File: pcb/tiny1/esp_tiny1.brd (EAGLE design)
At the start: 45 x 95 mm, 35 parts, among them IC1 4000D, Q1 BUZ11BH

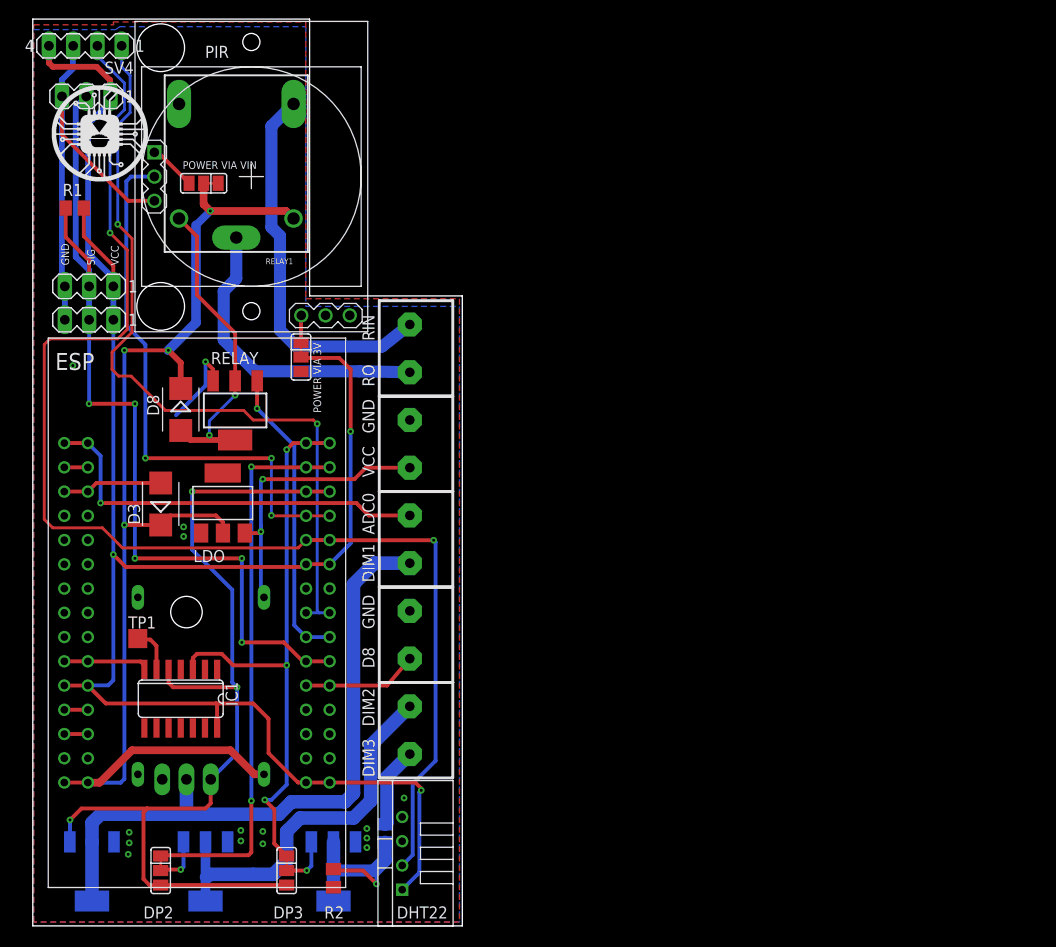
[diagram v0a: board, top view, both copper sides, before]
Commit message: added tiny board
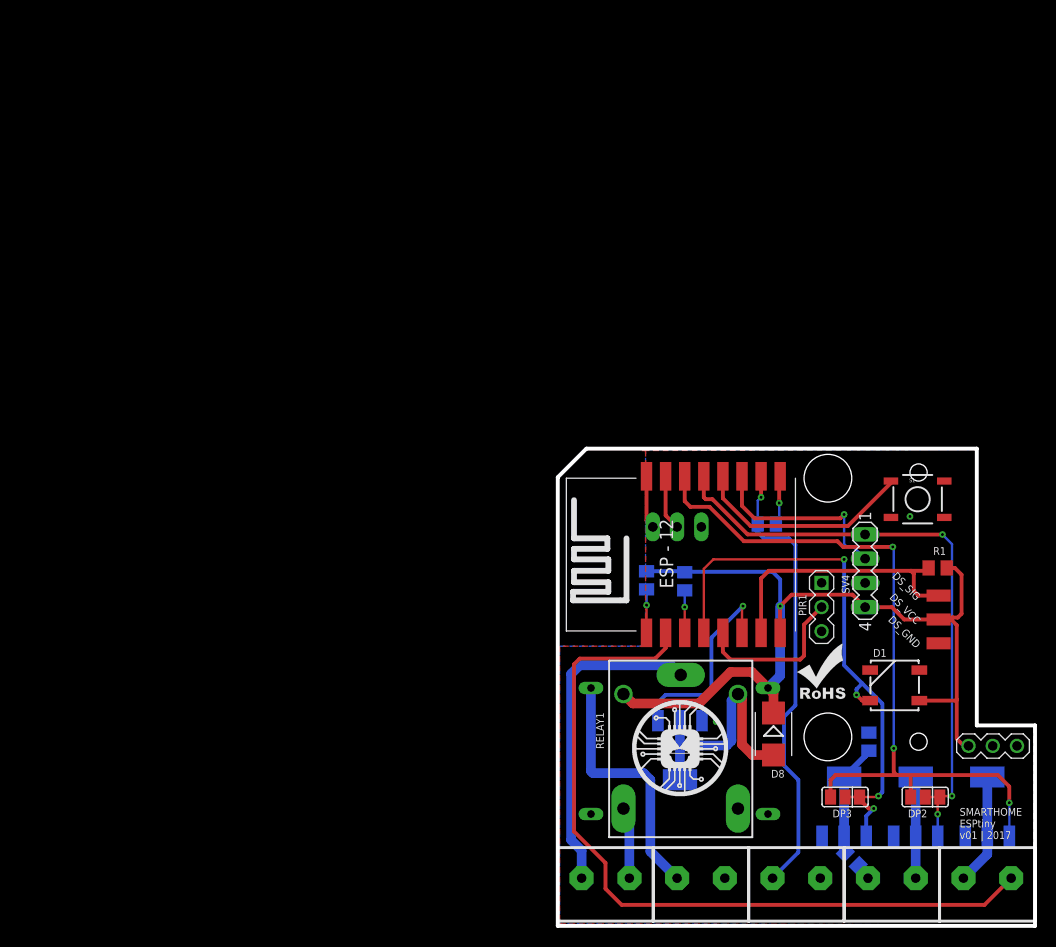
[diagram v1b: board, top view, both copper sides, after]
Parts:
- removed D3: ES2D, diode:SMB
- removed DHT22: TEMP-HUM-SENSOR-DHT22, diy-modules:TEMP-HUM-SENSOR-DHT22
- removed ESP: ESP12E_DEVKIT, ESP12E_DEVKIT:ESP12E_DEVKIT
- removed IC1: 4000D, 40xx:SO14
- removed LDO: REG1117, burr-brown:SOT223
- removed PIR: MOTION-PIR-DYP-ME003, diy-modules:MOTION-PIR-DYP-ME003
- removed Q1: BUZ11BH, transistor-power:TO220BH
- removed SV2, SV3: (no value), con-lstb:MA03-1
- removed TP1: TPTP20SQ, testpad:TP20SQ
- removed U$5, U$6: SMD_SJ_3WAY_CLOSED, JKW_CHIP:SMD_SJ_3WAY_CLOSED
- added D1: (no value), SparkFun-LED:WS2812B
- added DS_GND, DS_SIG, DS_VCC: (no value), wirepad:SMD1,27-2,54
- added PIR1: MOTION-PIR-DYP-ME003, diy-modules:MOTION-PIR-DYP-ME003_FRAMELESS
- added R4, R5, R6: 10k, rcl:M0805
- added S1: TAC_SWITCHSMD, SparkFun-Retired:TACTILE-SWITCH-SMD
- added U1: (no value), esp8266modules:ESP12-SMD
- U$12: value MP1584EN_FRAMELESS -> MP1584EN; device JKW_CHIP:MP1584EN_FRAMELESS -> JKW_CHIP:MP1584EN
- moved U$4 104.6 mm to (96.2, 22.7)
- moved SV4 98.5 mm to (87.2, 37.2), turned to 270 degrees
- moved R1 97.9 mm to (94.8, 37.5)
- moved T_DIM1 94.0 mm to (100.0, 12.5), turned to 0 degrees
- moved U$11 88.6 mm to (62.8, 13.6)
- moved U$9 85.8 mm to (79.6, 23.7), flipped to the top
- moved DP2 80.5 mm to (93.5, 13.5), turned to 180 degrees
- moved SV1 76.6 mm to (67.5, 41.8), flipped to the bottom, turned to 0 degrees
- moved RELAY1 76.6 mm to (68.0, 18.9), turned to 270 degrees
- moved T_DIM2 74.7 mm to (92.5, 12.5), turned to 0 degrees
- moved D8 70.8 mm to (77.6, 20.1)
- moved U$3 70.0 mm to (100.0, 4.50), turned to 0 degrees
- moved U$1 61.5 mm to (80.7, 28.9)
- moved U$8 59.5 mm to (60.0, 4.50), turned to 0 degrees
- moved DP3 59.0 mm to (85.1, 13.5), turned to 180 degrees
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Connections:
- removed net DIMM2: DP2.1, ESP.D1, ESP.D11
- removed net N$12: ESP.EN, ESP.EN1
- removed net N$13: ESP.RST, ESP.RST1
- removed net N$14: D3.A, ESP.RSV@1, ESP.RSV@11
- removed net N$24: PIR.4, U$5.1
- removed net N$31: PIR.1, U$6.3
- removed net PIR: ESP.D3, ESP.D31, PIR.2
- removed net RERLAY: ESP.D6, ESP.D61, RELAY.1
- new net A_IN: U$3.P$2, U1.ADC
- new net N$5: PIR1.2, U1.GPIO14
- new net N$6: SV1.2, U1.RXD0
- new net N$7: S1.1, U1.GPIO0
- new net RELAY: RELAY.1, U1.GPIO12
- net DHT_SIG/SDA: now also U1.GPIO2; no longer DHT22.2, ESP.D4, ESP.D41
- net DIMM1: now also U1.GPIO4; no longer ESP.D2, ESP.D21, IC1.5, Q1.G
- net DIMM3: now also D1.4, U1.GPIO16; no longer ESP.D0, ESP.D01, IC1.3
- net DIMMING1: no longer Q1.D
- net EARTH_HUM_POW: now also R5.1, U1.GPIO15; no longer ESP.D8, ESP.D81
- net GND: now also D1.3, DS_GND.1, PIR1.3, R5.2, S1.3, SV1.1, U1.GND; no longer DHT22.4, ESP.GND@0, ESP.GND@1, ESP.GND@2, ESP.GND@3, ESP.GND@4, ESP.GND@5, ESP.GND@6, ESP.GND@7, IC1.7, LDO.1, PIR.3, Q1.S, SV1.3, SV2.3, SV3.3
- net N$1: now also R6.1, U1.CH_PD; no longer ESP.AD0, ESP.AD1, U$3.P$2
- net N$17: no longer LDO.3
- net N$2: now also R4.1, U1.RESET; no longer ESP.RSV@0, ESP.RSV@01
- net N$4: now also SV1.3, U1.TXD0; no longer IC1.6, TP1.TP
- net ONEWIRE_DS12B20: now also DS_SIG.1, U1.GPIO13; no longer ESP.D7, ESP.D71, SV1.2, SV2.2, SV3.2
- net SCL: now also DP2.1, U1.GPIO5; no longer ESP.D5, ESP.D51
- net VCC: now also PIR1.1; no longer D3.C, D8.C, ESP.VIN, ESP.VIN1, LDO.2, RELAY1.COIL0, U$12.VOUT, U$6.2
- net VDD: now also D1.1, D8.C, DS_VCC.1, PIR1.4, R4.2, R6.2, RELAY1.COIL0, U$12.VOUT, U1.VCC; no longer DHT22.1, ESP.3V3@0, ESP.3V3@1, ESP.3V3@2, ESP.3V3@3, ESP.3V3@4, ESP.3V3@5, IC1.14, SV1.1, SV2.1, SV3.1, U$5.2
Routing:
- net VCC: track 123.5 -> 0.00 mm, vias 4 -> 0
- net DHT_SIG/SDA: track 138.4 -> 20.4 mm, vias 2 -> 1
- net VDD: track 194.7 -> 94.9 mm, vias 3 -> 1
- net A_IN: track 0.00 -> 81.1 mm
- net ONEWIRE_DS12B20: track 94.0 -> 28.7 mm, vias 5 -> 0
- net GND: track 64.1 -> 5.33 mm, vias 15 -> 3
- net PIR: track 58.3 -> 0.00 mm, vias 3 -> 0
- net DIMM2: track 58.3 -> 0.00 mm, vias 2 -> 0
- net DIMMING1: track 69.3 -> 11.6 mm
- net N$1: track 42.2 -> 4.45 mm
- net EARTH_HUM_POW: track 12.2 -> 47.8 mm, vias 0 -> 1
- net NORMALLY_OPEN: track 40.1 -> 7.55 mm
- net RERLAY: track 31.4 -> 0.00 mm, vias 1 -> 0
- net DIMMING2: track 40.4 -> 10.6 mm
- net SCL: track 82.5 -> 57.9 mm
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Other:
- board size 45 x 95 mm -> 50 x 50 mm
- board text added: "SMARTHOME ESPtiny v01 | 2017"
- board text removed: "DIM1"
- board text removed: "DIM2"
- board text removed: "DIM3"
- board text removed: "POWER VIA 3V"
- board text removed: "POWER VIA VIN"
- board text removed: "SIG"
- board text removed: "SMARTHOME ESP MQTT v03 | 2017"
